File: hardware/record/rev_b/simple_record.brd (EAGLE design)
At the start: 34.9 x 30 mm, 20 parts, among them J1 SQUALL_HEADER, J3 SCREW-TERMINAL_2_0.100, J4 SCREW-TERMINAL_2_0.100, Q1 MOSFET-NCHANNELSMD, U1 MAX9923T

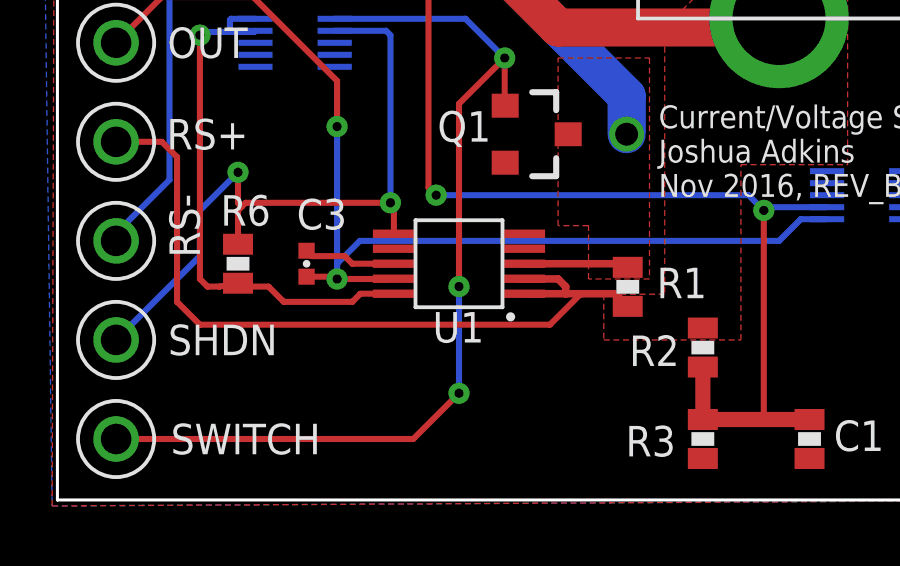
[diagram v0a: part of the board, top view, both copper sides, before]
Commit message: renumbered parts
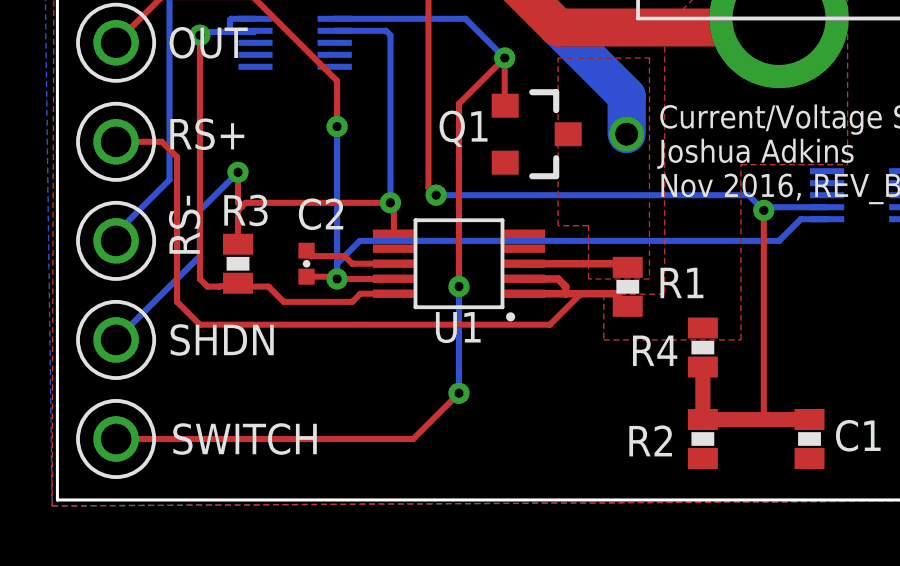
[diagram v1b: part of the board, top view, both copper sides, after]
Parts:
- removed R6: 100k, passives:0603-RES
- added R4: 176k, passives:0603-RES
- R2: value 176k -> 24k
- R3: value 24k -> 100k
- moved R3 16.6 mm to (-11.4, -4.83)
- moved R2 3.05 mm to (4.06, -10.7)
- renumbered C3 to C2
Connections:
- net GND: now also C2.2, R2.1; no longer C1.2, R3.1
- net N$7: now also C1.2; no longer C2.2
- net OUT: now also C1.1; no longer C2.1
- net PV+: now also R4.2; no longer R2.2
- net SHDN: now also R3.2; no longer R6.2
- net VCC: now also R3.1; no longer R6.1
- net VOUT: now also C2.1, R2.2, R4.1; no longer C1.1, R2.1, R3.2
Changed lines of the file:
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@@
 <setting verticaltext="up"/>
 </settings>
-<grid distance="0.01" unitdist="inch" unit="inch" style="lines" multiple="1" display="yes" altdistance="0.01" altunitdist="inch" altunit="inch"/>
+<grid distance="0.1" unitdist="inch" unit="inch" style="lines" multiple="1" display="yes" altdistance="0.01" altunitdist="inch" altunit="inch"/>
 <layers>
 <layer number="1" name="Top" color="4" fill="1" visible="yes" active="yes"/>
@@
 <attribute name="NAME" x="-3.89" y="-0.756" size="1.016" layer="25" font="vector" ratio="12" align="bottom-center"/>
 </element>
-<element name="R2" library="passives" package="0603-RES" value="176k" x="4.064" y="-7.62" smashed="yes" rot="R90">
+<element name="R4" library="passives" package="0603-RES" value="176k" x="4.064" y="-7.62" smashed="yes" rot="R90">
 <attribute name="NAME" x="2.448" y="-7.218" size="1.016" layer="25" font="vector" ratio="12" rot="R180" align="bottom-center"/>
 </element>
-<element name="R3" library="passives" package="0603-RES" value="24k" x="4.064" y="-10.668" smashed="yes" rot="R90">
+<element name="R2" library="passives" package="0603-RES" value="24k" x="4.064" y="-10.668" smashed="yes" rot="R90">
 <attribute name="NAME" x="2.326" y="-10.232" size="1.016" layer="25" font="vector" ratio="12" rot="R180" align="bottom-center"/>
 </element>
@@
 <attribute name="DIGIKEY" value="MAX9923HEUB+-ND" x="-4.064" y="-4.826" size="1.778" layer="27" font="vector" ratio="12" rot="R90" display="off"/>
 </element>
-<element name="C3" library="passives" package="0402_CAP" value="1nF" x="-9.144" y="-4.826" smashed="yes" rot="R90">
+<element name="C2" library="passives" package="0402_CAP" value="1nF" x="-9.144" y="-4.826" smashed="yes" rot="R90">
 <attribute name="NAME" x="-8.636" y="-2.667" size="1.016" layer="25" font="vector" ratio="12" rot="R180" align="bottom-center"/>
 </element>
-<element name="R6" library="passives" package="0603-RES" value="100k" x="-11.43" y="-4.826" smashed="yes" rot="R90">
+<element name="R3" library="passives" package="0603-RES" value="100k" x="-11.43" y="-4.826" smashed="yes" rot="R90">
 <attribute name="NAME" x="-11.176" y="-2.54" size="1.016" layer="25" font="vector" ratio="12" rot="R180" align="bottom-center"/>
 </element>
@@
 <signal name="GND">
 <contactref element="Q1" pad="2"/>
-<contactref element="R3" pad="1"/>
-<contactref element="C1" pad="2"/>
+<contactref element="R2" pad="1"/>
+<contactref element="C2" pad="2"/>
 <contactref element="J1" pad="A9"/>
 <contactref element="J1" pad="A10"/>
@@
 </signal>
 <signal name="PV+">
-<contactref element="R2" pad="2"/>
+<contactref element="R4" pad="2"/>
 <contactref element="R1" pad="2"/>
 <contactref element="TP5" pad="TESTPOINT"/>
@@
 <wire x1="-10.885" y1="2.9" x2="-10.845" y2="2.94" width="0.2032" layer="16"/>
 <contactref element="U1" pad="10"/>
-<contactref element="R6" pad="1"/>
+<contactref element="R3" pad="1"/>
 <wire x1="-6.234" y1="-5.826" x2="-7.35" y2="-5.826" width="0.2032" layer="1"/>
 <wire x1="-7.35" y1="-5.826" x2="-7.62" y2="-6.096" width="0.2032" layer="1"/>
@@
 </signal>
 <signal name="VOUT">
-<contactref element="R2" pad="1"/>
-<contactref element="R3" pad="2"/>
-<contactref element="C1" pad="1"/>
+<contactref element="R4" pad="1"/>
+<contactref element="R2" pad="2"/>
+<contactref element="C2" pad="1"/>
 <contactref element="J1" pad="B7"/>
 <contactref element="TP4" pad="TESTPOINT"/>
@@
 <signal name="OUT">
 <contactref element="U1" pad="9"/>
-<contactref element="C3" pad="1"/>
+<contactref element="C1" pad="1"/>
 <contactref element="J1" pad="B9"/>
 <contactref element="TP7" pad="TESTPOINT"/>
@@
 <signal name="N$7">
 <contactref element="U1" pad="8"/>
-<contactref element="C3" pad="2"/>
+<contactref element="C1" pad="2"/>
 <wire x1="-6.234" y1="-4.826" x2="-7.62" y2="-4.826" width="0.2032" layer="1"/>
 <wire x1="-7.62" y1="-4.826" x2="-7.874" y2="-4.572" width="0.2032" layer="1"/>
@@
 <signal name="SHDN">
 <contactref element="U1" pad="6"/>
-<contactref element="R6" pad="2"/>
+<contactref element="R3" pad="2"/>
 <contactref element="TP1" pad="TESTPOINT"/>
 <contactref element="J1" pad="A4"/>

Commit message: Revert "renumbered parts"
This reverts commit aba0891c6fa3a8957b5f6f1ce6d6696c13dad33f.

Something wonky happened there. I sure hope that commit message is
accurate and nothing else was changed...
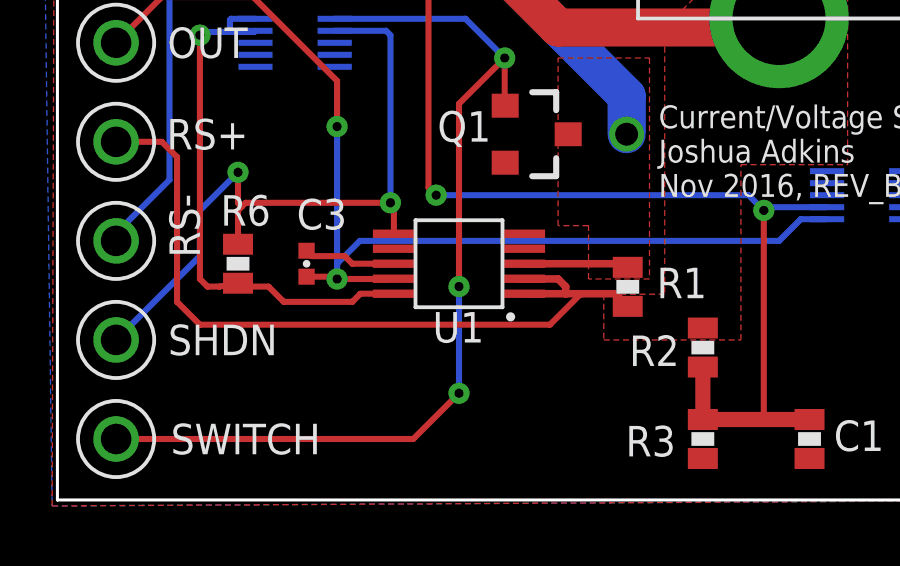
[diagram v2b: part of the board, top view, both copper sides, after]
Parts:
- removed R4: 176k, passives:0603-RES
- added R6: 100k, passives:0603-RES
- R2: value 24k -> 176k
- R3: value 100k -> 24k
- moved R3 16.6 mm to (4.06, -10.7)
- moved R2 3.05 mm to (4.06, -7.62)
- renumbered C2 to C3
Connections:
- net GND: now also C1.2, R3.1; no longer C3.2, R2.1
- net N$7: now also C3.2; no longer C1.2
- net OUT: now also C3.1; no longer C1.1
- net PV+: now also R2.2; no longer R4.2
- net SHDN: now also R6.2; no longer R3.2
- net VCC: now also R6.1; no longer R3.1
- net VOUT: now also C1.1, R2.1, R3.2; no longer C3.1, R2.2, R4.1
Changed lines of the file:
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@@
 <setting verticaltext="up"/>
 </settings>
-<grid distance="0.1" unitdist="inch" unit="inch" style="lines" multiple="1" display="yes" altdistance="0.01" altunitdist="inch" altunit="inch"/>
+<grid distance="0.01" unitdist="inch" unit="inch" style="lines" multiple="1" display="yes" altdistance="0.01" altunitdist="inch" altunit="inch"/>
 <layers>
 <layer number="1" name="Top" color="4" fill="1" visible="yes" active="yes"/>
@@
 <attribute name="NAME" x="-3.89" y="-0.756" size="1.016" layer="25" font="vector" ratio="12" align="bottom-center"/>
 </element>
-<element name="R4" library="passives" package="0603-RES" value="176k" x="4.064" y="-7.62" smashed="yes" rot="R90">
+<element name="R2" library="passives" package="0603-RES" value="176k" x="4.064" y="-7.62" smashed="yes" rot="R90">
 <attribute name="NAME" x="2.448" y="-7.218" size="1.016" layer="25" font="vector" ratio="12" rot="R180" align="bottom-center"/>
 </element>
-<element name="R2" library="passives" package="0603-RES" value="24k" x="4.064" y="-10.668" smashed="yes" rot="R90">
+<element name="R3" library="passives" package="0603-RES" value="24k" x="4.064" y="-10.668" smashed="yes" rot="R90">
 <attribute name="NAME" x="2.326" y="-10.232" size="1.016" layer="25" font="vector" ratio="12" rot="R180" align="bottom-center"/>
 </element>
@@
 <attribute name="DIGIKEY" value="MAX9923HEUB+-ND" x="-4.064" y="-4.826" size="1.778" layer="27" font="vector" ratio="12" rot="R90" display="off"/>
 </element>
-<element name="C2" library="passives" package="0402_CAP" value="1nF" x="-9.144" y="-4.826" smashed="yes" rot="R90">
+<element name="C3" library="passives" package="0402_CAP" value="1nF" x="-9.144" y="-4.826" smashed="yes" rot="R90">
 <attribute name="NAME" x="-8.636" y="-2.667" size="1.016" layer="25" font="vector" ratio="12" rot="R180" align="bottom-center"/>
 </element>
-<element name="R3" library="passives" package="0603-RES" value="100k" x="-11.43" y="-4.826" smashed="yes" rot="R90">
+<element name="R6" library="passives" package="0603-RES" value="100k" x="-11.43" y="-4.826" smashed="yes" rot="R90">
 <attribute name="NAME" x="-11.176" y="-2.54" size="1.016" layer="25" font="vector" ratio="12" rot="R180" align="bottom-center"/>
 </element>
@@
 <signal name="GND">
 <contactref element="Q1" pad="2"/>
-<contactref element="R2" pad="1"/>
-<contactref element="C2" pad="2"/>
+<contactref element="R3" pad="1"/>
+<contactref element="C1" pad="2"/>
 <contactref element="J1" pad="A9"/>
 <contactref element="J1" pad="A10"/>
@@
 </signal>
 <signal name="PV+">
-<contactref element="R4" pad="2"/>
+<contactref element="R2" pad="2"/>
 <contactref element="R1" pad="2"/>
 <contactref element="TP5" pad="TESTPOINT"/>
@@
 <wire x1="-10.885" y1="2.9" x2="-10.845" y2="2.94" width="0.2032" layer="16"/>
 <contactref element="U1" pad="10"/>
-<contactref element="R3" pad="1"/>
+<contactref element="R6" pad="1"/>
 <wire x1="-6.234" y1="-5.826" x2="-7.35" y2="-5.826" width="0.2032" layer="1"/>
 <wire x1="-7.35" y1="-5.826" x2="-7.62" y2="-6.096" width="0.2032" layer="1"/>
@@
 </signal>
 <signal name="VOUT">
-<contactref element="R4" pad="1"/>
-<contactref element="R2" pad="2"/>
-<contactref element="C2" pad="1"/>
+<contactref element="R2" pad="1"/>
+<contactref element="R3" pad="2"/>
+<contactref element="C1" pad="1"/>
 <contactref element="J1" pad="B7"/>
 <contactref element="TP4" pad="TESTPOINT"/>
@@
 <signal name="OUT">
 <contactref element="U1" pad="9"/>
-<contactref element="C1" pad="1"/>
+<contactref element="C3" pad="1"/>
 <contactref element="J1" pad="B9"/>
 <contactref element="TP7" pad="TESTPOINT"/>
@@
 <signal name="N$7">
 <contactref element="U1" pad="8"/>
-<contactref element="C1" pad="2"/>
+<contactref element="C3" pad="2"/>
 <wire x1="-6.234" y1="-4.826" x2="-7.62" y2="-4.826" width="0.2032" layer="1"/>
 <wire x1="-7.62" y1="-4.826" x2="-7.874" y2="-4.572" width="0.2032" layer="1"/>
@@
 <signal name="SHDN">
 <contactref element="U1" pad="6"/>
-<contactref element="R3" pad="2"/>
+<contactref element="R6" pad="2"/>
 <contactref element="TP1" pad="TESTPOINT"/>
 <contactref element="J1" pad="A4"/>
